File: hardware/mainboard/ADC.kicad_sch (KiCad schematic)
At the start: 19 parts, among them IC8 ADC 24bit, IC9 LTC1799

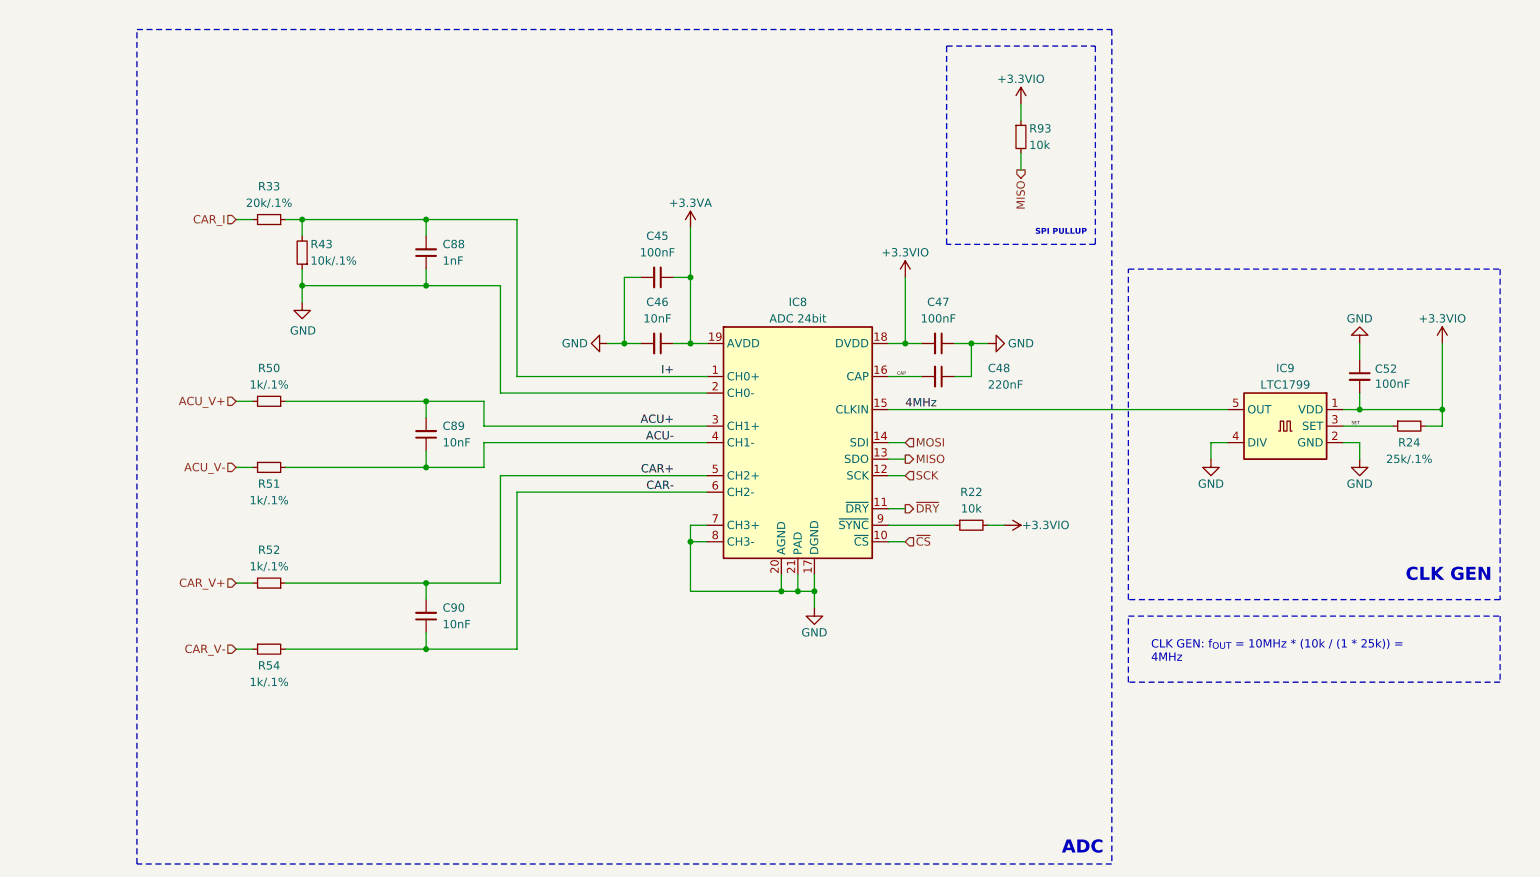
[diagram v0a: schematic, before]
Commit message: isolation with every thing
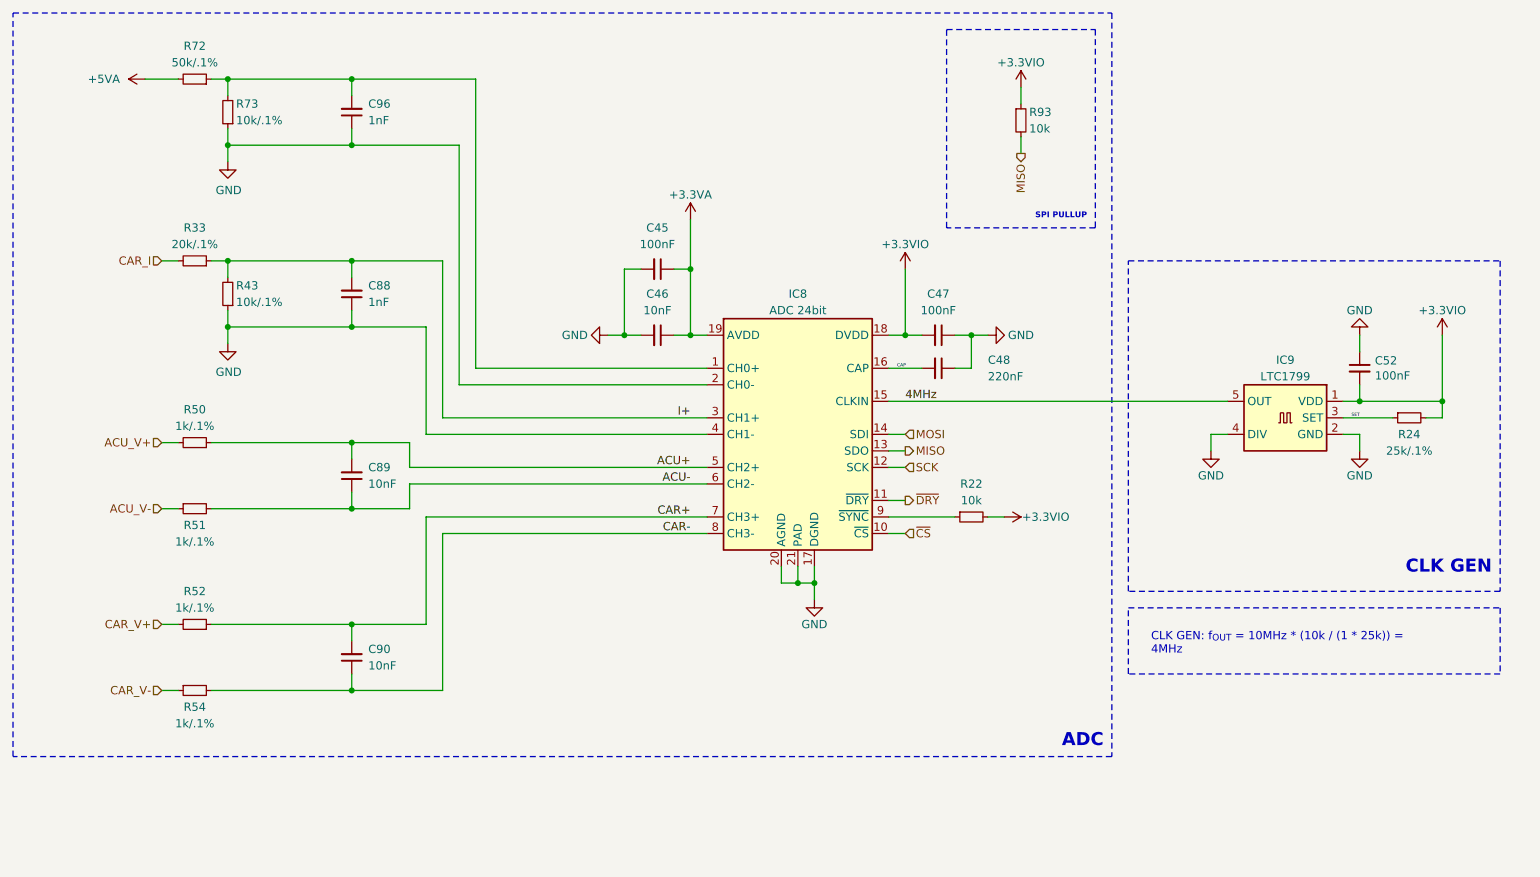
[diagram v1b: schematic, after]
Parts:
- added C96: 1nF, Capacitor_SMD:C_0603_1608Metric, symbol Device:C_Small
- added R72: 50k/.1%, Resistor_SMD:R_0603_1608Metric, symbol Device:R_Small
- added R73: 10k/.1%, Resistor_SMD:R_0603_1608Metric, symbol Device:R_Small
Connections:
- net ACU+: now also IC8.5 (CH2+); no longer IC8.3 (CH1+)
- net ACU-: now also IC8.6 (CH2-); no longer IC8.4 (CH1-)
- net CAR+: now also IC8.7 (CH3+); no longer IC8.5 (CH2+)
- net CAR-: now also IC8.8 (CH3-); no longer IC8.6 (CH2-)
- net GND: now also IC8.4 (CH1-), C96.1, R73.1; no longer IC8.7 (CH3+), IC8.8 (CH3-)
- net I+: now also IC8.3 (CH1+); no longer IC8.1 (CH0+)
- new net: C96.2, IC8.1 (CH0+), R72.1, R73.2
- new net +5VA: R72.2
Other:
- moved on the sheet: C45, C46, C47, C48, C52, C88, C89, C90, IC8, IC9, R22, R24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
